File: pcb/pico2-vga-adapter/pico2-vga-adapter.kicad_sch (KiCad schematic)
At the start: 71 parts, among them J1 USB_B_Micro, J2 VGA, J3 CONN, J4 SM03B-SRSS-TB, J5 Conn_01x08_Pin, J6 UART, Q1 BSS138, Q10 BSS138, Q2 BSS138, Q3 BSS138, Q4 BSS138, Q5 BSS138, Q6 BSS138, Q7 BSS138, Q8 BSS138, Q9 BSS138, SW1 SW_Push, SW2 SW_Push, U1 RP2350_60QFN, U2 NCP1117-3.3_SOT223, U3 W25Q128JVS, Y1 ABM8-272-T3

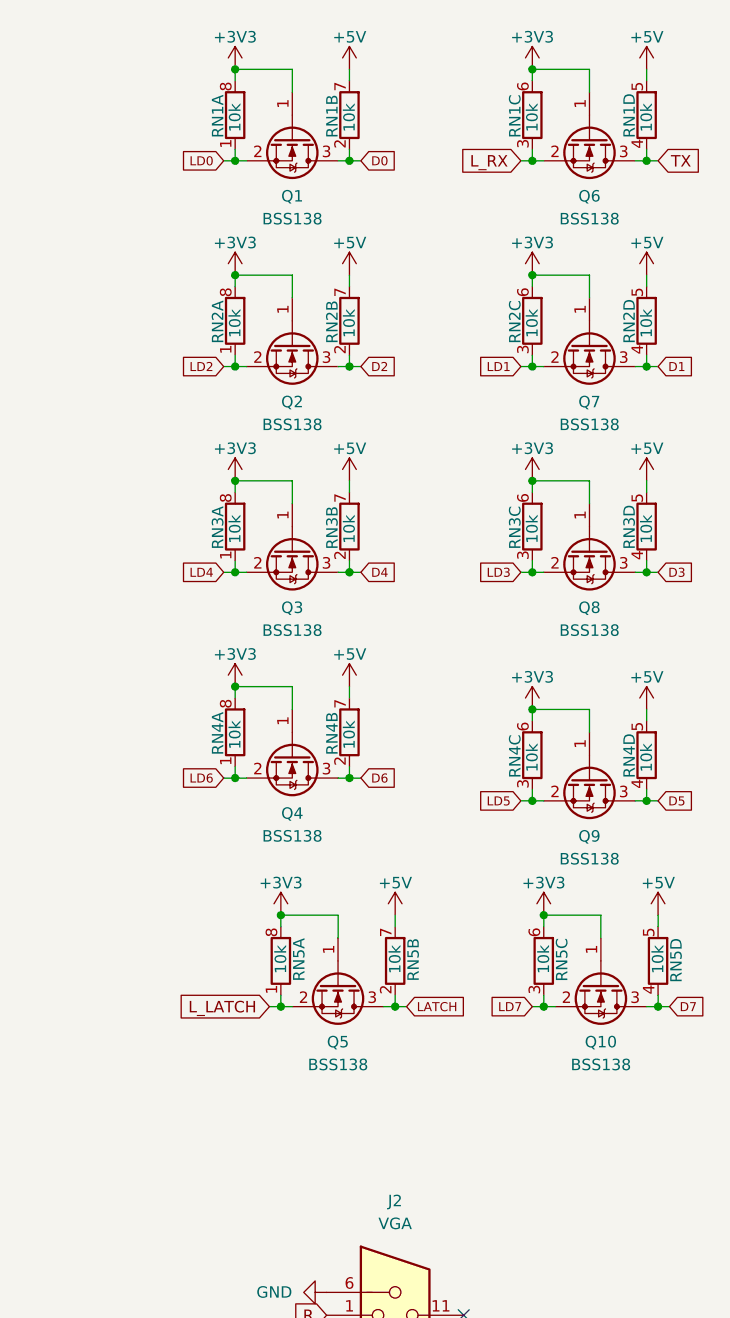
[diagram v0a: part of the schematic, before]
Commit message: Routing
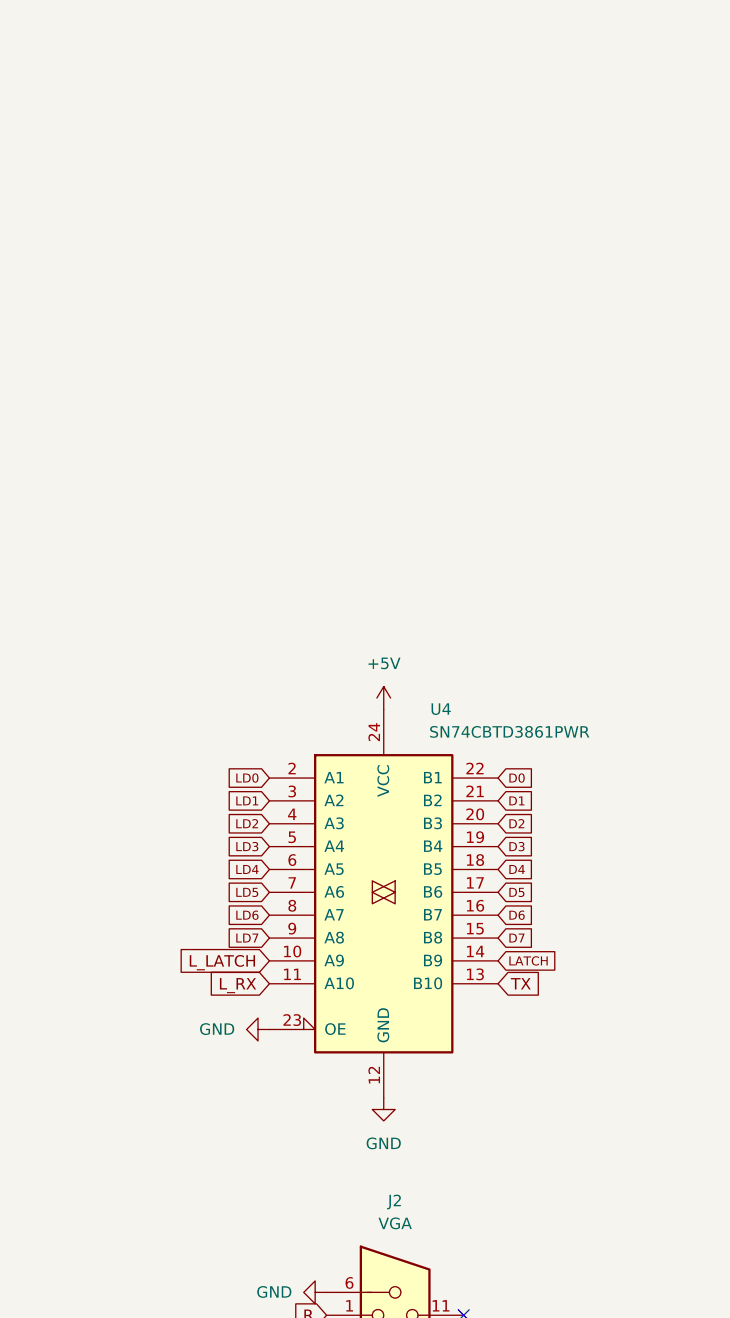
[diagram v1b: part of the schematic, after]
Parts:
- removed Q1, Q10, Q2, Q3, Q4, Q5, Q6, Q7, Q8, Q9: BSS138, Package_TO_SOT_SMD:SOT-23, symbol Transistor_FET:BSS138
- removed RN1, RN2, RN3, RN4, RN5: 10k, Resistor_SMD:R_Array_Convex_4x0603, symbol Device:R_Pack04_Split
- added U4: SN74CBTD3861PWR, Package_SO:TSSOP-24_4.4x7.8mm_P0.65mm, symbol vera-module-rev4-rescue:74CBTLV3861-74xx
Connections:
- net +5V: now also U4.24 (VCC)
- net D0: now also U4.22 (B1)
- net D1: now also U4.21 (B2)
- net D2: now also U4.20 (B3)
- net D3: now also U4.19 (B4)
- net D4: now also U4.18 (B5)
- net D5: now also U4.17 (B6)
- net D6: now also U4.16 (B7)
- net D7: now also U4.15 (B8)
- net GND: now also U4.12 (GND), U4.23 (OE)
- net LATCH: now also U4.14 (B9)
- net LD0: now also U4.2 (A1)
- net LD1: now also U4.3 (A2)
- net LD2: now also U4.4 (A3)
- net LD3: now also U4.5 (A4)
- net LD4: now also U4.6 (A5)
- net LD5: now also U4.7 (A6)
- net LD6: now also U4.8 (A7)
- net LD7: now also U4.9 (A8)
- net L_LATCH: now also U4.10 (A9)
- net L_RX: now also U4.11 (A10)
- net TX: now also U4.13 (B10)
